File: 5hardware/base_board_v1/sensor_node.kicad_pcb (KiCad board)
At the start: 2 copper layers, 24.5 x 49.6 mm, 21 parts, among them J1 Conn_01x06_Pin, J2 Conn_01x08_Pin, J3 Conn_01x09_Pin, J4 USB_C_Receptacle_USB2.0, P1 USB_C_Plug_USB2.0, SW1 SW_Push, SW2 SW_Push, SW7 SW_Push, U1 ESP-12F, U2 CH32V003F4P6, U3 XC6206PxxxMR

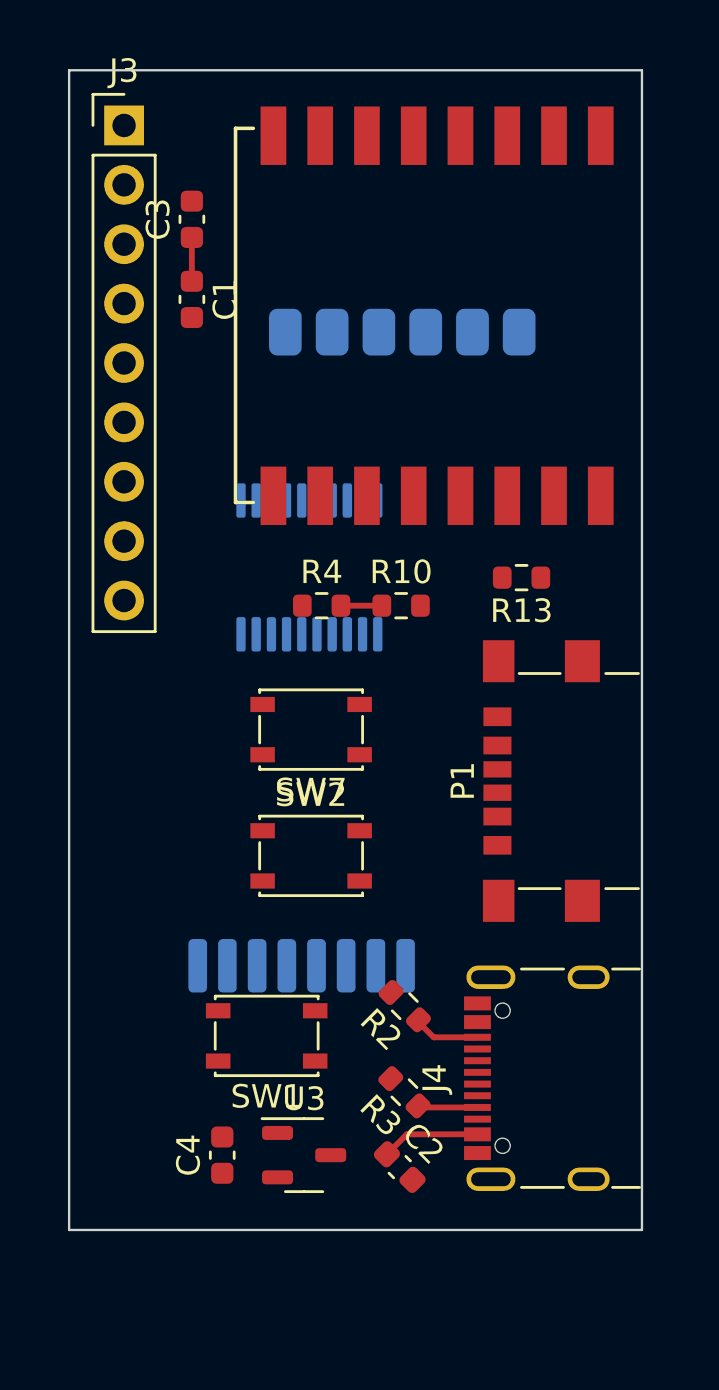
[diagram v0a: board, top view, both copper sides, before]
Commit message: update pcb.
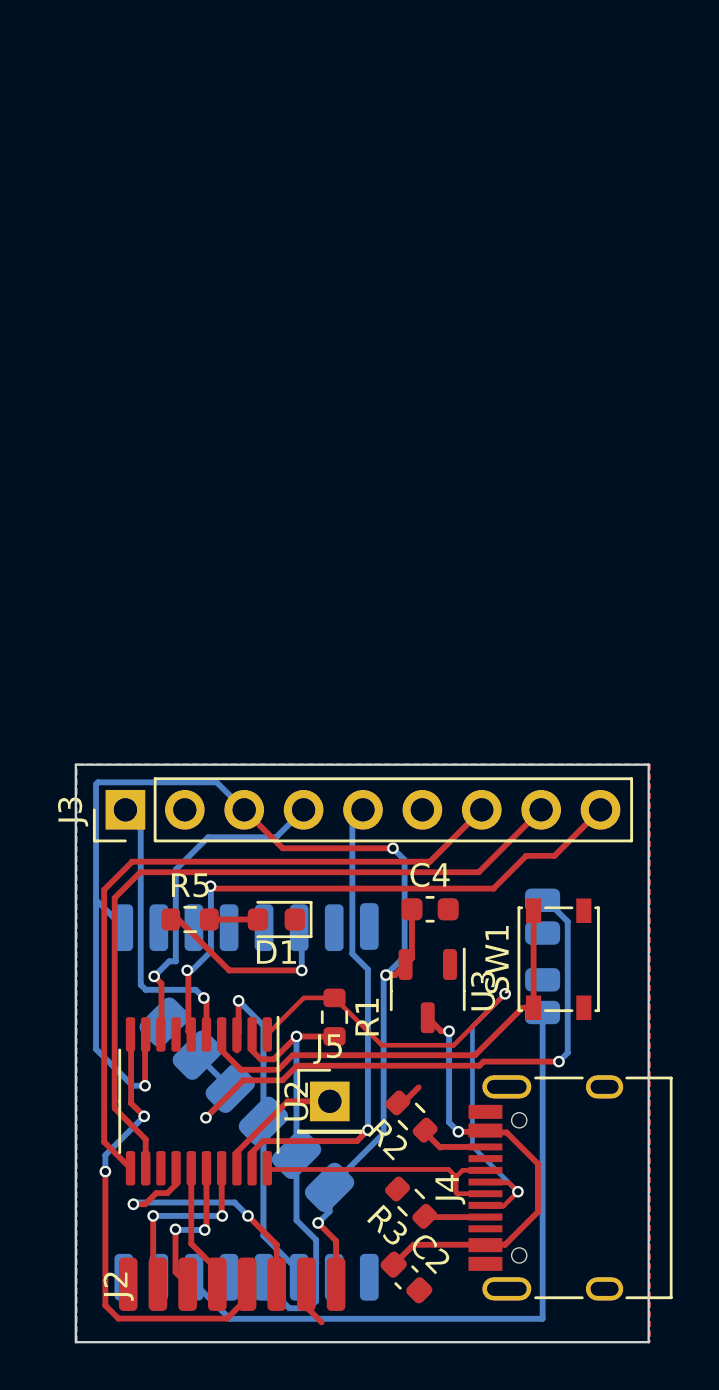
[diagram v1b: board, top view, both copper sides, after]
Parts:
- removed C1, C3: C, Capacitor_SMD:C_0603_1608Metric
- removed P1: USB_C_Plug_USB2.0, Connector_USB:USB_C_Receptacle_GCT_USB4135-GF-A_6P_TopMnt_Horizontal
- removed R10, R13: R, Resistor_SMD:R_0603_1608Metric
- removed SW2, SW7: SW_Push, Button_Switch_SMD:SW_SPST_PTS810
- removed U1: ESP-12F, A_SensorNode:ESP12_SMD
- added D1: LED, LED_SMD:LED_0603_1608Metric, F.Cu at (144.4, 94.7)
- added J5: Conn_01x01_Pin, Connector_PinHeader_2.54mm:PinHeader_1x01_P2.54mm_Vertical, F.Cu at (146.7, 102.5)
- added R1: R, Resistor_SMD:R_0603_1608Metric, F.Cu at (146.9, 98.9)
- added R5: R, Resistor_SMD:R_0603_1608Metric, F.Cu at (140.7, 94.7)
- added R6: 0K, A_SensorNode:Jumpper, B.Cu at (155.8, 93.9)
- added U4: ~, A_SensorNode:JDY-Base, B.Cu at (149.9, 110.0)
- J2, U2: moved to F.Cu
- J4: footprint Connector_USB:USB_C_Receptacle_GCT_USB4105-xx-A_16P_TopMnt_Horizontal -> Connector_USB:USB_C_Receptacle_HRO_TYPE-C-31-M-12
- R4: value R -> 0K; footprint Resistor_SMD:R_0603_1608Metric -> A_SensorNode:Jumpper; moved to B.Cu
- moved J1 73.8 mm to (122.7, 113.2), turned to -45 degrees
- moved J3 29.3 mm to (138.0, 90.0), turned to 90 degrees
- moved G*** 27.6 mm to (152.2, 68.8), turned to 90 degrees
- moved U2 23.3 mm to (141.1, 102.5)
- moved R4 18.6 mm to (155.8, 97.3), turned to -90 degrees
- moved J2 18.1 mm to (138.1, 110.3)
- moved C4 13.8 mm to (151.0, 94.3), turned to 0 degrees
- moved SW1 12.9 mm to (156.5, 96.4), turned to 90 degrees
- moved U3 8.79 mm to (150.9, 97.8), turned to -90 degrees
- moved J4 4.74 mm to (157.4, 106.2)
- moved C2 4.73 mm to (150.0, 110.0)
- moved R2 4.73 mm to (150.2, 103.1)
- moved R3 4.73 mm to (150.2, 106.8)
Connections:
- net Vi+ renamed V+
- J1 pad 1: +3.3V -> GND
- J1 pad 2: RX -> CON2
- J1 pad 3: TX -> CON2
- J1 pad 4: unconnected-(J1-Pin_4-Pad4) -> RX
- J1 pad 5: unconnected-(J1-Pin_5-Pad5) -> TX
- J1 pad 6: GND -> +3.3V
- J2 pad 1: +3.3V -> unconnected-(J2-Pin_1-Pad1)
- J2 pad 2: GND -> MISO
- J2 pad 3: CE -> MOSI
- J2 pad 4: CS -> SCK
- J2 pad 5: SCK -> CS
- J2 pad 6: MOSI -> CE
- J2 pad 7: MISO -> GND
- J2 pad 8: unconnected-(J2-Pin_8-Pad8) -> +3.3V
- R4 pad 1: EN1 -> GND
- R4 pad 2: +3.3V -> CON1
- U2 pad 2: RX -> TX
- U2 pad 3: TX -> RX
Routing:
- net +3.3V: track 3.72 -> 55.4 mm, vias 0 -> 4
- net SCL: track 0.00 -> 31.9 mm
- net SDA: track 0.00 -> 29.9 mm
- net CON1: track 0.00 -> 28.9 mm
- net CON2: track 0.00 -> 27.4 mm, vias 0 -> 2
- net D-: track 0.00 -> 25.7 mm, vias 0 -> 2
- net SW-B: track 0.00 -> 24.8 mm, vias 0 -> 2
- net DONE: track 0.00 -> 20.9 mm, vias 0 -> 1
- net CS: track 0.00 -> 19.8 mm, vias 0 -> 2
- net Net-(U2-PD7): track 0.00 -> 19.6 mm
- net TX: track 0.00 -> 19.5 mm, vias 0 -> 1
- net RX: track 0.00 -> 15.1 mm, vias 0 -> 1
- net Net-(U3-VI): track 4.23 -> 18.7 mm, vias 0 -> 2
- net DRIVE: track 0.00 -> 14.3 mm, vias 0 -> 1
- net SW-A: track 0.00 -> 12.3 mm, vias 0 -> 1
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- added copper zone on B.Cu, net GND
- added copper zone on F.Cu, net GND
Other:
- board size 24.5 x 49.6 mm -> 24.5 x 24.7 mm
